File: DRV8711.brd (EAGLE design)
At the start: 66.5 x 53.5 mm, 37 parts, among them IC1 DRV8711, T1 IPC50N04S5, T2 IPC50N04S5, T3 IPC50N04S5, T4 IPC50N04S5, T5 IPC50N04S5, T6 IPC50N04S5, T7 IPC50N04S5, T8 IPC50N04S5

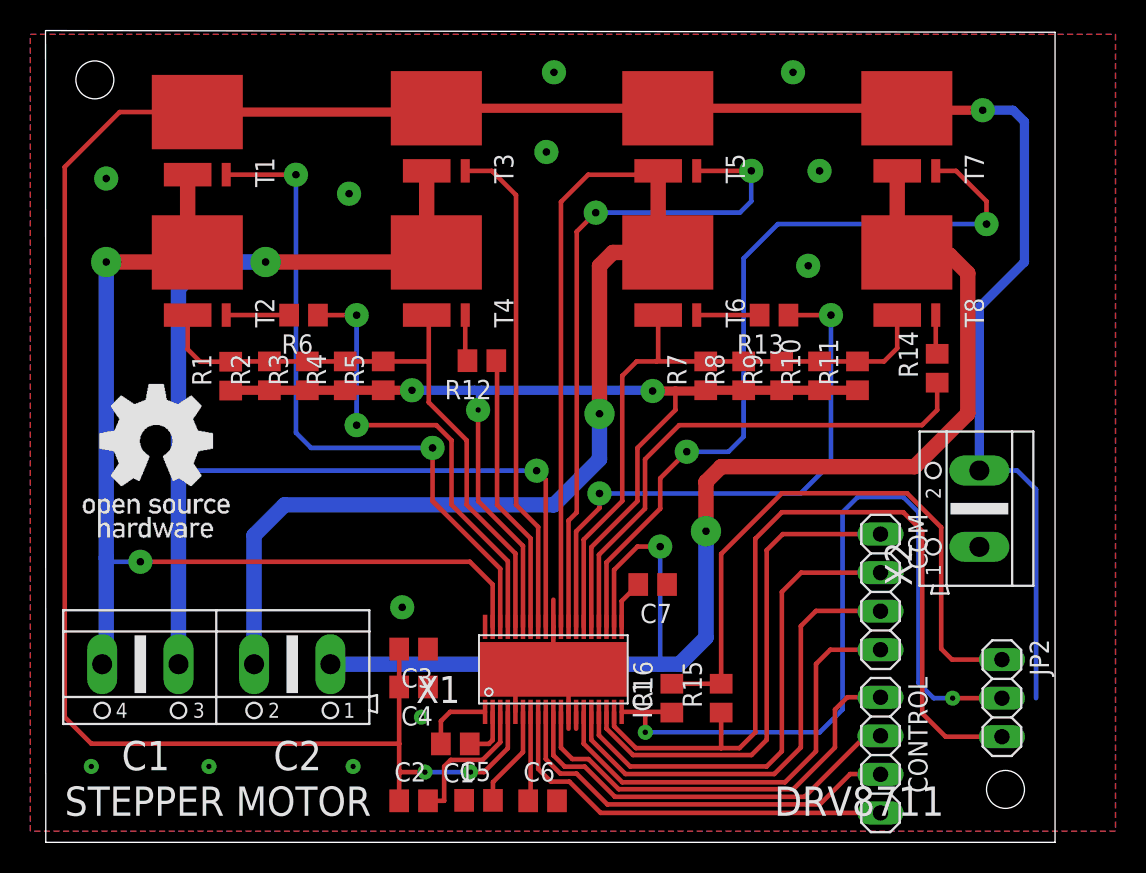
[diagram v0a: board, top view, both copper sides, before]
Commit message: Add files via upload
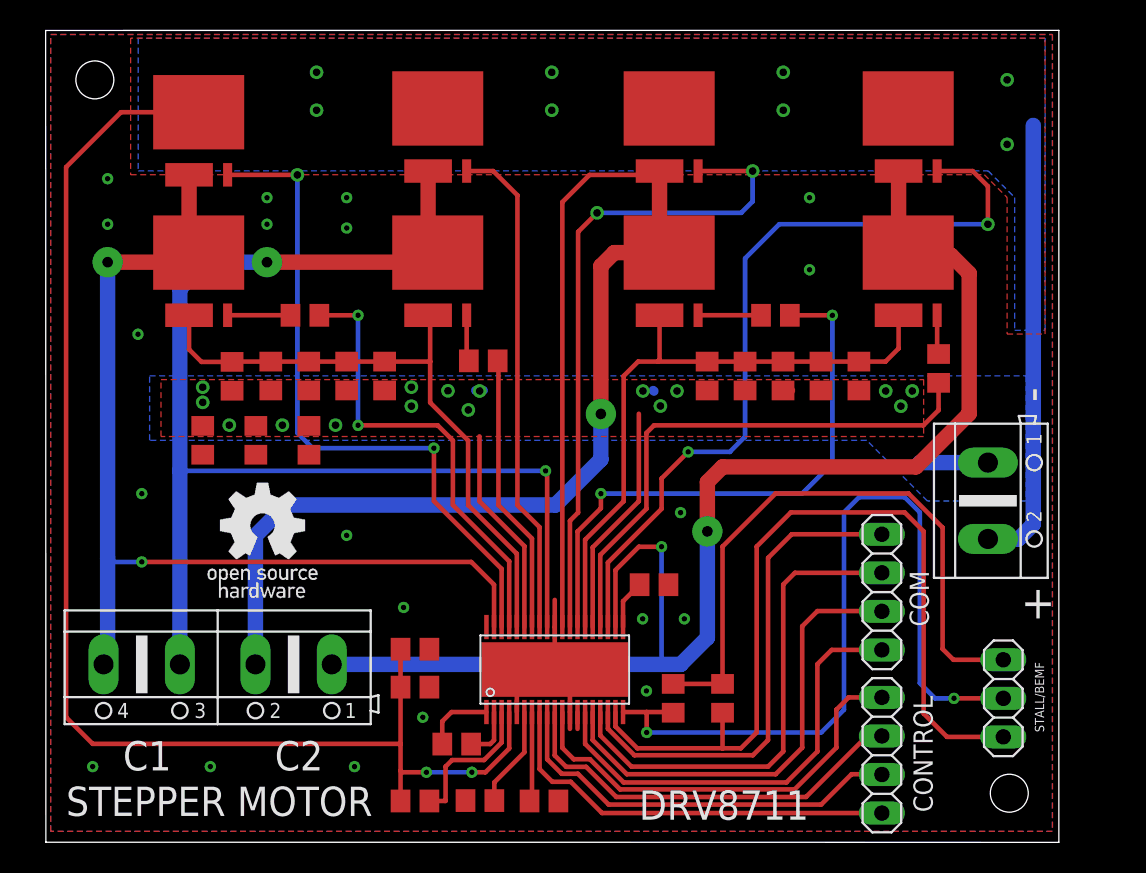
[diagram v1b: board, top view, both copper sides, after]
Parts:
- removed JP2: (no value), pinhead:1X03
- added R17, R18, R19: 0R, rcl:R0805
- added STALL/BEMF: (no value), pinhead:1X03
- moved X2 0.77 mm to (62.1, 22.5), turned to 270 degrees
- moved COM 0.09 mm to (55.1, 16.5)
- moved CONTROL 0.09 mm to (55.1, 5.74)
- moved IC1 0.09 mm to (33.5, 11.4)
- moved R15 0.09 mm to (44.6, 9.49)
- moved R16 0.09 mm to (41.3, 9.49)
- moved C3 0.09 mm to (24.3, 12.7)
- moved C4 0.09 mm to (24.3, 10.2)
- moved X1 0.09 mm to (11.3, 11.7)
- moved C5 0.09 mm to (28.6, 2.75)
- moved C1 0.09 mm to (27.1, 6.48)
- moved C2 0.09 mm to (24.3, 2.73)
- moved R1 0.09 mm to (12.3, 30.7)
- moved R12 0.09 mm to (28.8, 31.7)
- moved R2 0.09 mm to (14.8, 30.7)
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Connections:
- net +5V: now also STALL/BEMF.1; no longer JP2.1
- net AGND: now also R17.1, R18.1, R19.1, X2.1
- net FAULT: now also STALL/BEMF.3; no longer JP2.3
- net GND: now also R17.2, R18.2, R19.2; no longer X2.1
- net STALL: now also STALL/BEMF.2; no longer JP2.2
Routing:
- net V+: track 187.6 -> 123.3 mm, vias 3 -> 10
- net AGND: track 79.5 -> 35.1 mm, vias 3 -> 16
- net B2LS: track 34.7 -> 35.7 mm
- net B2HS: track 52.3 -> 52.8 mm
- net GND: vias 12 -> 20
- added copper zone on layer 1, net AGND
- added copper zone on layer 16, net AGND
- added copper zone on layer 1, net V+
- added copper zone on layer 16, net V+
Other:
- board size 66.5 x 53.5 mm -> 66.8 x 53.5 mm
- board text added: "+"
- board text added: "-"
